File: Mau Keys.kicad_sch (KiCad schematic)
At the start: 36 parts

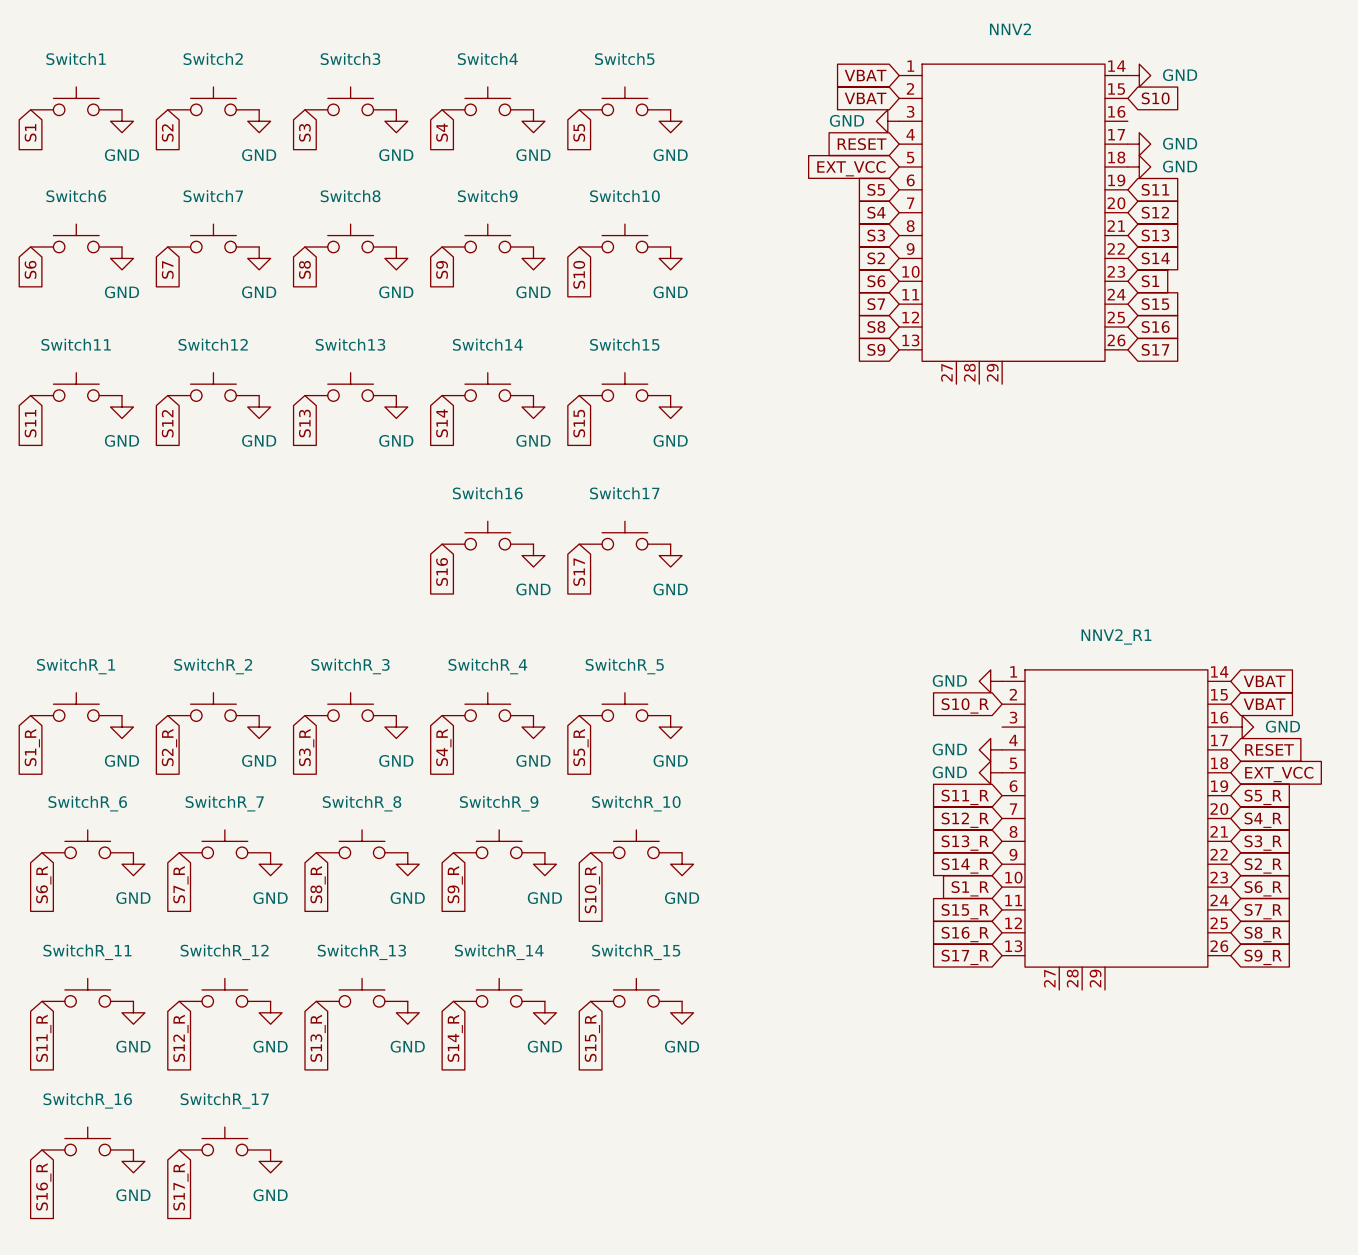
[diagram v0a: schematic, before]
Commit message: Traces upper left
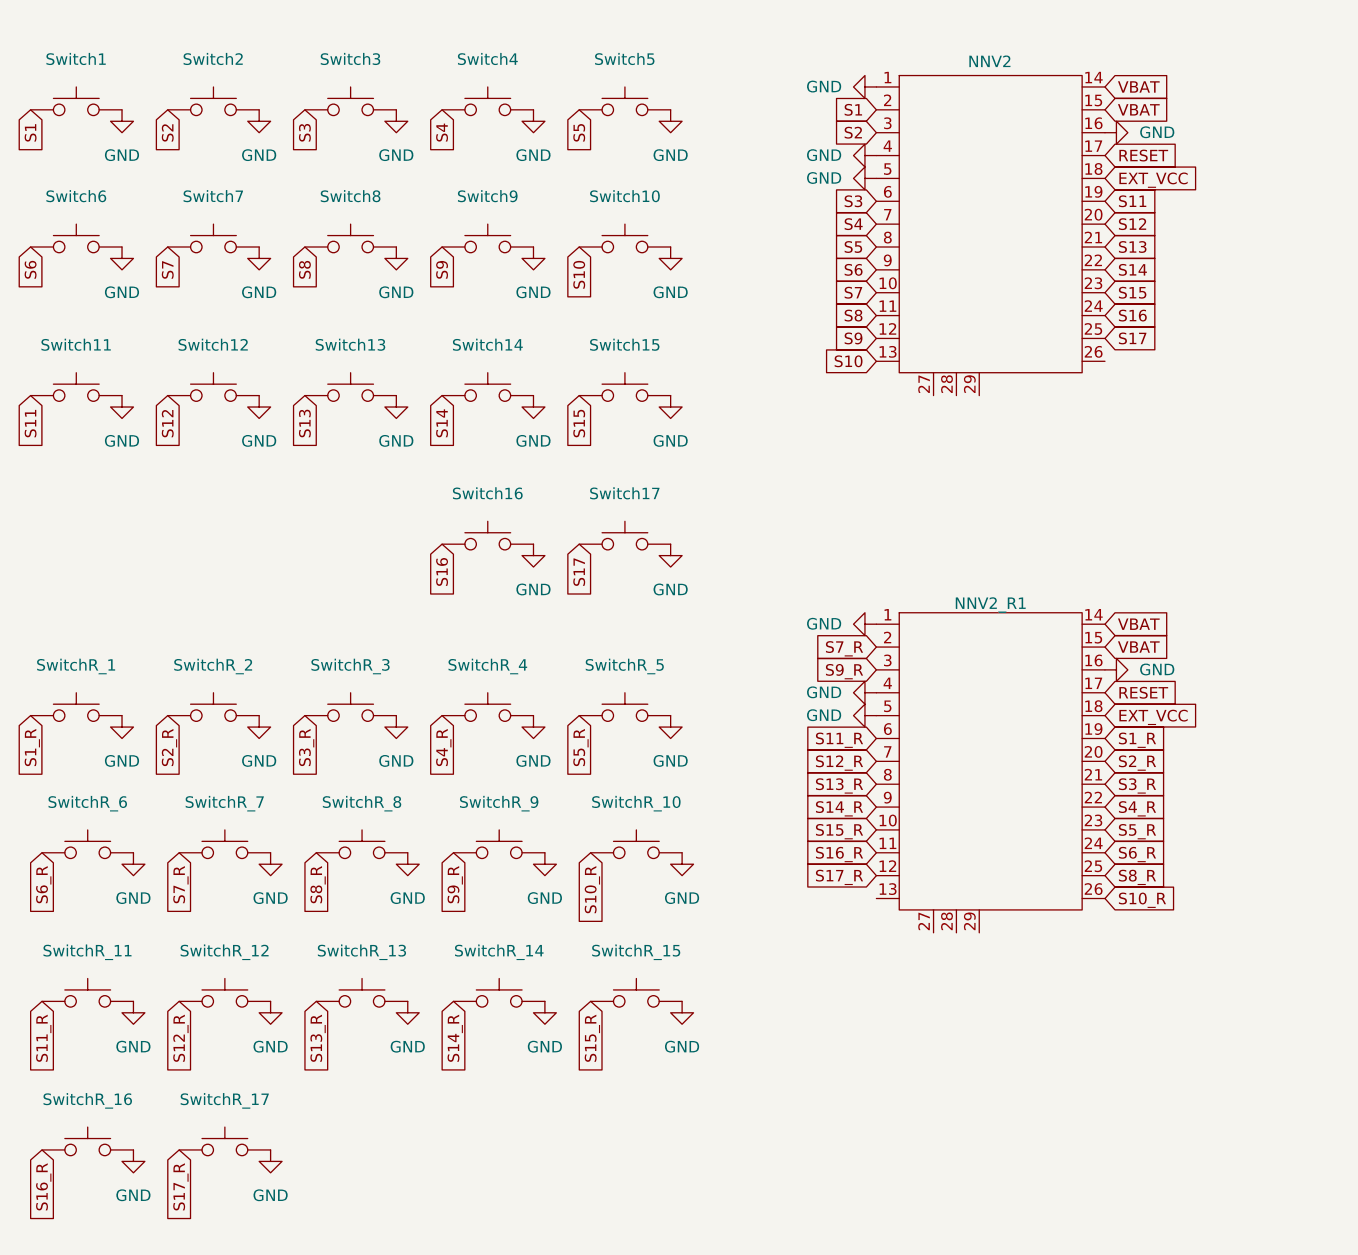
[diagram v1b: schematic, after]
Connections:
- net EXT_VCC: now also NNV2.18; no longer NNV2.5
- net GND: now also NNV2.1, NNV2.16, NNV2.4, NNV2.5; no longer NNV2.14, NNV2.17, NNV2.18, NNV2.3
- net RESET: now also NNV2.17; no longer NNV2.4
- net S1: now also NNV2.2; no longer NNV2.23
- net S10: now also NNV2.13; no longer NNV2.15
- net S10_R: now also NNV2_R1.26; no longer NNV2_R1.2
- net S15: now also NNV2.23; no longer NNV2.24
- net S15_R: now also NNV2_R1.10; no longer NNV2_R1.11
- net S16: now also NNV2.24; no longer NNV2.25
- net S16_R: now also NNV2_R1.11; no longer NNV2_R1.12
- net S17: now also NNV2.25; no longer NNV2.26
- net S17_R: now also NNV2_R1.12; no longer NNV2_R1.13
- net S1_R: now also NNV2_R1.19; no longer NNV2_R1.10
- net S2: now also NNV2.3; no longer NNV2.9
- net S2_R: now also NNV2_R1.20; no longer NNV2_R1.22
- net S3: now also NNV2.6; no longer NNV2.8
- net S4_R: now also NNV2_R1.22; no longer NNV2_R1.20
- net S5: now also NNV2.8; no longer NNV2.6
- net S5_R: now also NNV2_R1.23; no longer NNV2_R1.19
- net S6: now also NNV2.9; no longer NNV2.10
- net S6_R: now also NNV2_R1.24; no longer NNV2_R1.23
- net S7: now also NNV2.10; no longer NNV2.11
- net S7_R: now also NNV2_R1.2; no longer NNV2_R1.24
- net S8: now also NNV2.11; no longer NNV2.12
- net S9: now also NNV2.12; no longer NNV2.13
- net S9_R: now also NNV2_R1.3; no longer NNV2_R1.26
- net VBAT: now also NNV2.14, NNV2.15; no longer NNV2.1, NNV2.2
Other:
- moved on the sheet: NNV2, NNV2_R1
